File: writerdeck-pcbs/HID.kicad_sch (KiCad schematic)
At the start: 22 parts, among them SW2 SW_Push, SW3 SW_MEC_5E, U3 RP2040, U4 W25Q16JVSS, Y1 X322512MSB4SI

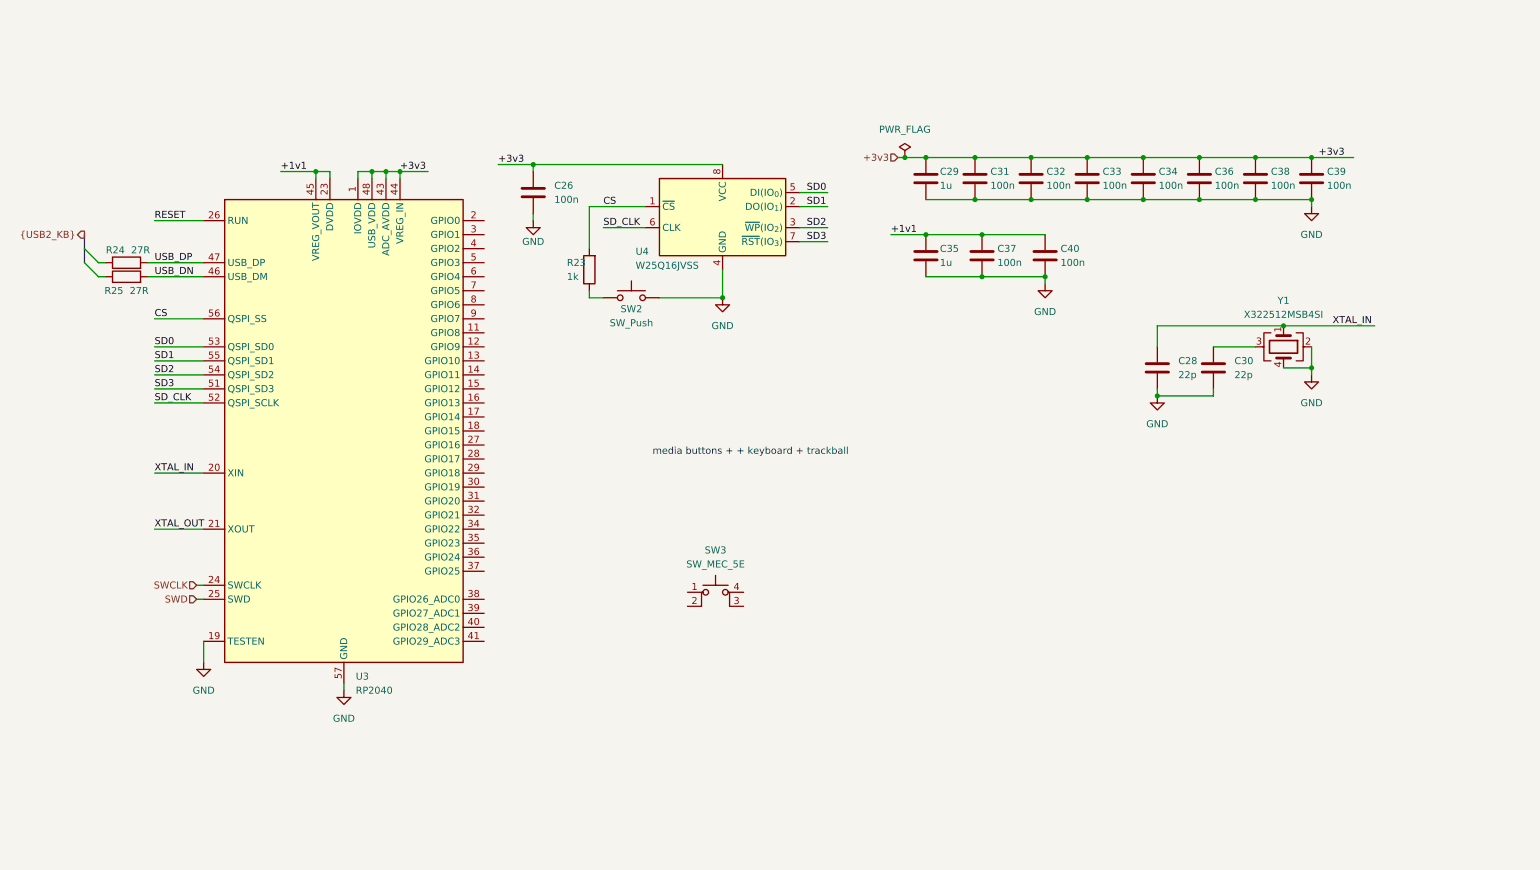
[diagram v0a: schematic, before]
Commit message: backup
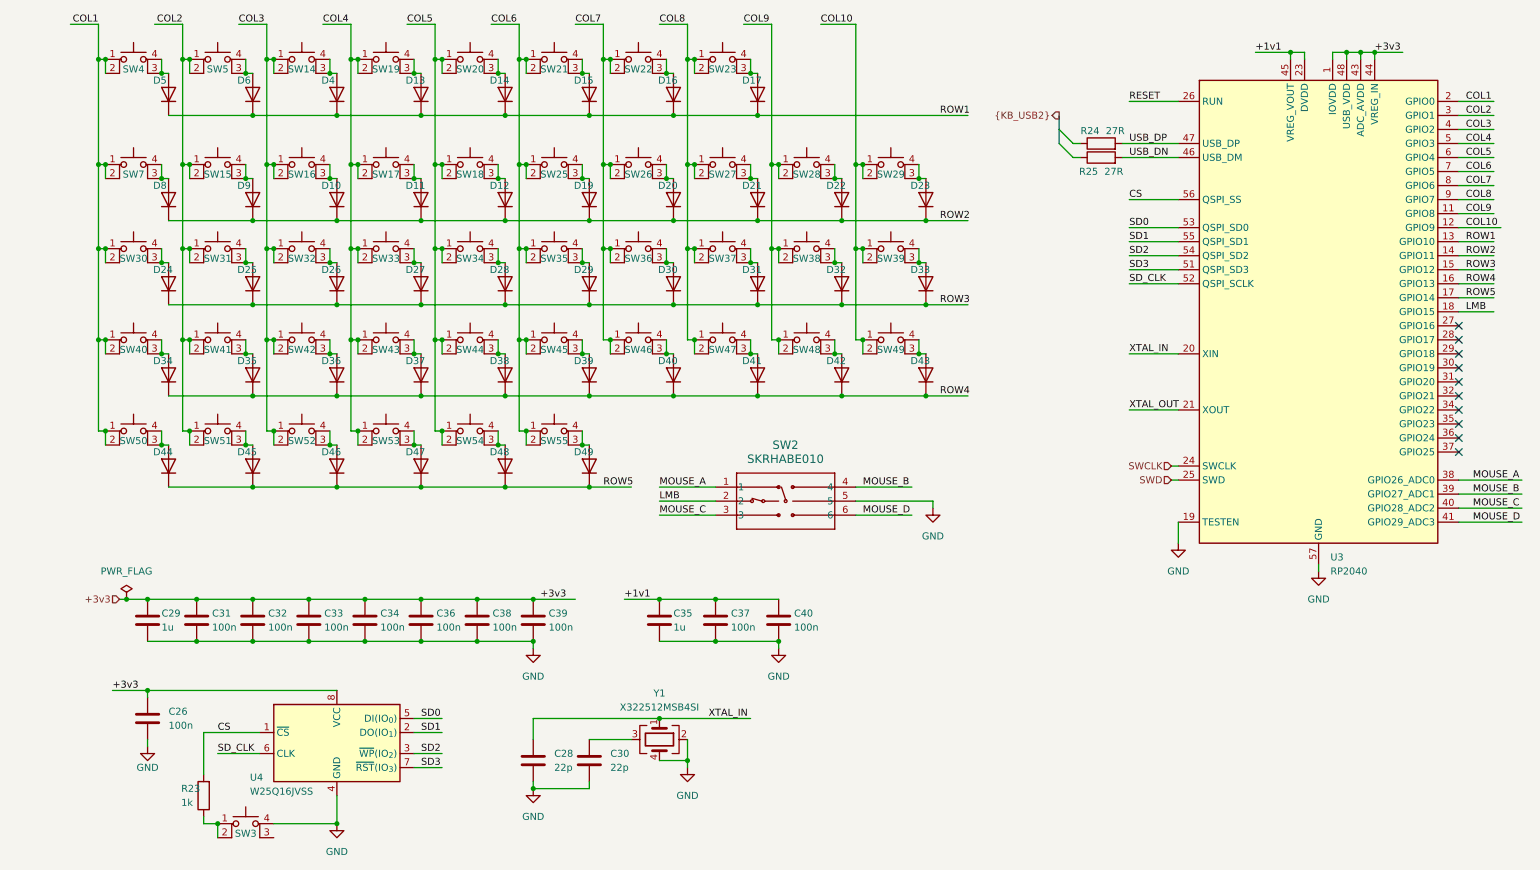
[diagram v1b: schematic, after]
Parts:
- removed SW2: SW_Push, symbol Switch:SW_Push
- removed SW3: SW_MEC_5E, symbol Switch:SW_MEC_5E
- added D10, D11, D12, D13, D14, D15, D16, D17, D19, D20, D21, D22, D23, D24, D25, D26, D27, D28, D29, D30, D31, D32, D33, D34, D35, D36, D37, D38, D39, D4, D40, D41, D42, D43, D44, D45, D46, D47, D48, D49, D5, D6, D8, D9: 1N4148W-TP, Diode_SMD:D_SOD-123, symbol ZF_common:1N4148W-TP
- added SW14, SW15, SW16, SW17, SW18, SW19, SW20, SW21, SW22, SW23, SW25, SW26, SW27, SW28, SW29, SW3, SW30, SW31, SW32, SW33, SW34, SW35, SW36, SW37, SW38, SW39, SW4, SW40, SW41, SW42, SW43, SW44, SW45, SW46, SW47, SW48, SW49, SW5, SW50, SW51, SW52, SW53, SW54, SW55, SW7: Tact Switch, symbol ZF_common:Tact Switch
- added SW2: SKRHABE010, ZF_common:SKRHABE010, symbol ZF_common:SKRHABE010
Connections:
- net GND: now also SW2.5, SW3.4 (A)
- net at R23.1: now also SW3.1, SW3.2
- net COL9: now reaches U3.11 (GPIO8)
- net COL9: now also SW28.1, SW28.2, SW38.1, SW38.2, SW48.1, SW48.2
- net COL10: now reaches U3.12 (GPIO9)
- net COL10: now also SW29.1, SW29.2, SW39.1, SW39.2, SW49.1, SW49.2
- net ROW1: now reaches U3.13 (GPIO10)
- net ROW1: now also D13.1 (K), D14.1 (K), D15.1 (K), D16.1 (K), D17.1 (K), D4.1 (K), D5.1 (K), D6.1 (K)
- net ROW2: now reaches U3.14 (GPIO11)
- net ROW2: now also D10.1 (K), D11.1 (K), D12.1 (K), D19.1 (K), D20.1 (K), D21.1 (K), D22.1 (K), D23.1 (K), D8.1 (K), D9.1 (K)
- net ROW3: now reaches U3.15 (GPIO12)
- net ROW3: now also D24.1 (K), D25.1 (K), D26.1 (K), D27.1 (K), D28.1 (K), D29.1 (K), D30.1 (K), D31.1 (K), D32.1 (K), D33.1 (K)
- net ROW4: now reaches U3.16 (GPIO13)
- net ROW4: now also D34.1 (K), D35.1 (K), D36.1 (K), D37.1 (K), D38.1 (K), D39.1 (K), D40.1 (K), D41.1 (K), D42.1 (K), D43.1 (K)
- net ROW5: now reaches U3.17 (GPIO14)
- net ROW5: now also D44.1 (K), D45.1 (K), D46.1 (K), D47.1 (K), D48.1 (K), D49.1 (K)
- net LMB: now reaches U3.18 (GPIO15)
- net LMB: now also SW2.2
- net COL1: now reaches U3.2 (GPIO0)
- net COL1: now also SW30.1, SW30.2, SW4.1, SW4.2, SW40.1, SW40.2, SW50.1, SW50.2, SW7.1, SW7.2
- net COL2: now reaches U3.3 (GPIO1)
- net COL2: now also SW15.1, SW15.2, SW31.1, SW31.2, SW41.1, SW41.2, SW5.1, SW5.2, SW51.1, SW51.2
- net MOUSE_A: now reaches U3.38 (GPIO26_ADC0)
- net MOUSE_A: now also SW2.1
- net MOUSE_B: now reaches U3.39 (GPIO27_ADC1)
- net MOUSE_B: now also SW2.4
- net COL3: now reaches U3.4 (GPIO2)
- net COL3: now also SW14.1, SW14.2, SW16.1, SW16.2, SW32.1, SW32.2, SW42.1, SW42.2, SW52.1, SW52.2
- net MOUSE_C: now reaches U3.40 (GPIO28_ADC2)
- net MOUSE_C: now also SW2.3
- net MOUSE_D: now reaches U3.41 (GPIO29_ADC3)
- net MOUSE_D: now also SW2.6
- net COL4: now reaches U3.5 (GPIO3)
- net COL4: now also SW17.1, SW17.2, SW19.1, SW19.2, SW33.1, SW33.2, SW43.1, SW43.2, SW53.1, SW53.2
- net COL5: now reaches U3.6 (GPIO4)
- net COL5: now also SW18.1, SW18.2, SW20.1, SW20.2, SW34.1, SW34.2, SW44.1, SW44.2, SW54.1, SW54.2
- net COL6: now reaches U3.7 (GPIO5)
- net COL6: now also SW21.1, SW21.2, SW25.1, SW25.2, SW35.1, SW35.2, SW45.1, SW45.2, SW55.1, SW55.2
- net COL7: now reaches U3.8 (GPIO6)
- net COL7: now also SW22.1, SW22.2, SW26.1, SW26.2, SW36.1, SW36.2, SW46.1, SW46.2
- net COL8: now reaches U3.9 (GPIO7)
- net COL8: now also SW23.1, SW23.2, SW27.1, SW27.2, SW37.1, SW37.2, SW47.1, SW47.2
- new net: D9.2 (A), SW15.3 (K), SW15.4 (A)
- new net: D39.2 (A), SW45.3 (K), SW45.4 (A)
- new net: D41.2 (A), SW47.3 (K), SW47.4 (A)
- new net: D10.2 (A), SW16.3 (K), SW16.4 (A)
- new net: D16.2 (A), SW22.3 (K), SW22.4 (A)
- new net: D24.2 (A), SW30.3 (K), SW30.4 (A)
- new net: D17.2 (A), SW23.3 (K), SW23.4 (A)
- new net: D13.2 (A), SW19.3 (K), SW19.4 (A)
- new net: D32.2 (A), SW38.3 (K), SW38.4 (A)
- new net: D43.2 (A), SW49.3 (K), SW49.4 (A)
- new net: D44.2 (A), SW50.3 (K), SW50.4 (A)
- new net: D46.2 (A), SW52.3 (K), SW52.4 (A)
- new net: D31.2 (A), SW37.3 (K), SW37.4 (A)
- new net: D6.2 (A), SW5.3 (K), SW5.4 (A)
- new net: D4.2 (A), SW14.3 (K), SW14.4 (A)
- new net: D45.2 (A), SW51.3 (K), SW51.4 (A)
- new net: D47.2 (A), SW53.3 (K), SW53.4 (A)
- new net: D23.2 (A), SW29.3 (K), SW29.4 (A)
- new net: D20.2 (A), SW26.3 (K), SW26.4 (A)
- new net: D34.2 (A), SW40.3 (K), SW40.4 (A)
- new net: D36.2 (A), SW42.3 (K), SW42.4 (A)
- new net: D14.2 (A), SW20.3 (K), SW20.4 (A)
- new net: D11.2 (A), SW17.3 (K), SW17.4 (A)
- new net: D37.2 (A), SW43.3 (K), SW43.4 (A)
- new net: D48.2 (A), SW54.3 (K), SW54.4 (A)
- new net: D25.2 (A), SW31.3 (K), SW31.4 (A)
- new net: D22.2 (A), SW28.3 (K), SW28.4 (A)
- new net: D28.2 (A), SW34.3 (K), SW34.4 (A)
- new net: D21.2 (A), SW27.3 (K), SW27.4 (A)
- new net: D26.2 (A), SW32.3 (K), SW32.4 (A)
- new net: D5.2 (A), SW4.3 (K), SW4.4 (A)
- new net: D15.2 (A), SW21.3 (K), SW21.4 (A)
- new net: D35.2 (A), SW41.3 (K), SW41.4 (A)
- new net: D49.2 (A), SW55.3 (K), SW55.4 (A)
- new net: D8.2 (A), SW7.3 (K), SW7.4 (A)
- new net: D30.2 (A), SW36.3 (K), SW36.4 (A)
- new net: D19.2 (A), SW25.3 (K), SW25.4 (A)
- new net: D40.2 (A), SW46.3 (K), SW46.4 (A)
- new net: D38.2 (A), SW44.3 (K), SW44.4 (A)
- new net: D33.2 (A), SW39.3 (K), SW39.4 (A)
- new net: D27.2 (A), SW33.3 (K), SW33.4 (A)
- new net: D29.2 (A), SW35.3 (K), SW35.4 (A)
- new net: D12.2 (A), SW18.3 (K), SW18.4 (A)
- new net: D42.2 (A), SW48.3 (K), SW48.4 (A)
- no-connect marks 0 -> 10
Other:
- note removed: "media buttons + + keyboard + trackball"
- moved on the sheet: C26, C28, C29, C30, C31, C32, C33, C34, C35, C36, C37, C38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
